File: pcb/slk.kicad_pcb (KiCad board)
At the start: 2 copper layers, 68.6 x 53.3 mm, 15 parts, among them J1 Screw Terminal, P1 Power, P2 Analog, P3 Digital 1, P4 Digital 2, U1 MCP2515-xSO, U2 TJA1055T1, Y1 Crystal

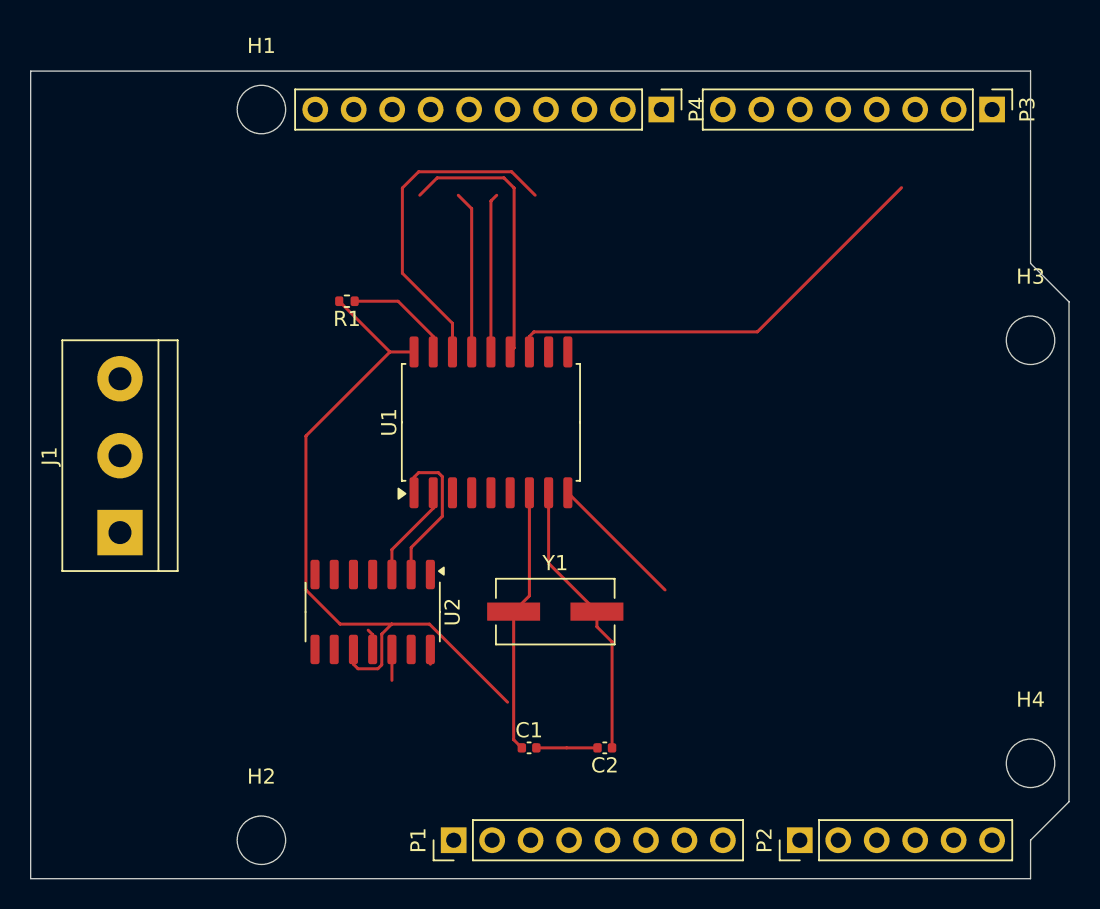
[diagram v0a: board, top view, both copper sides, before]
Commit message: it should work now
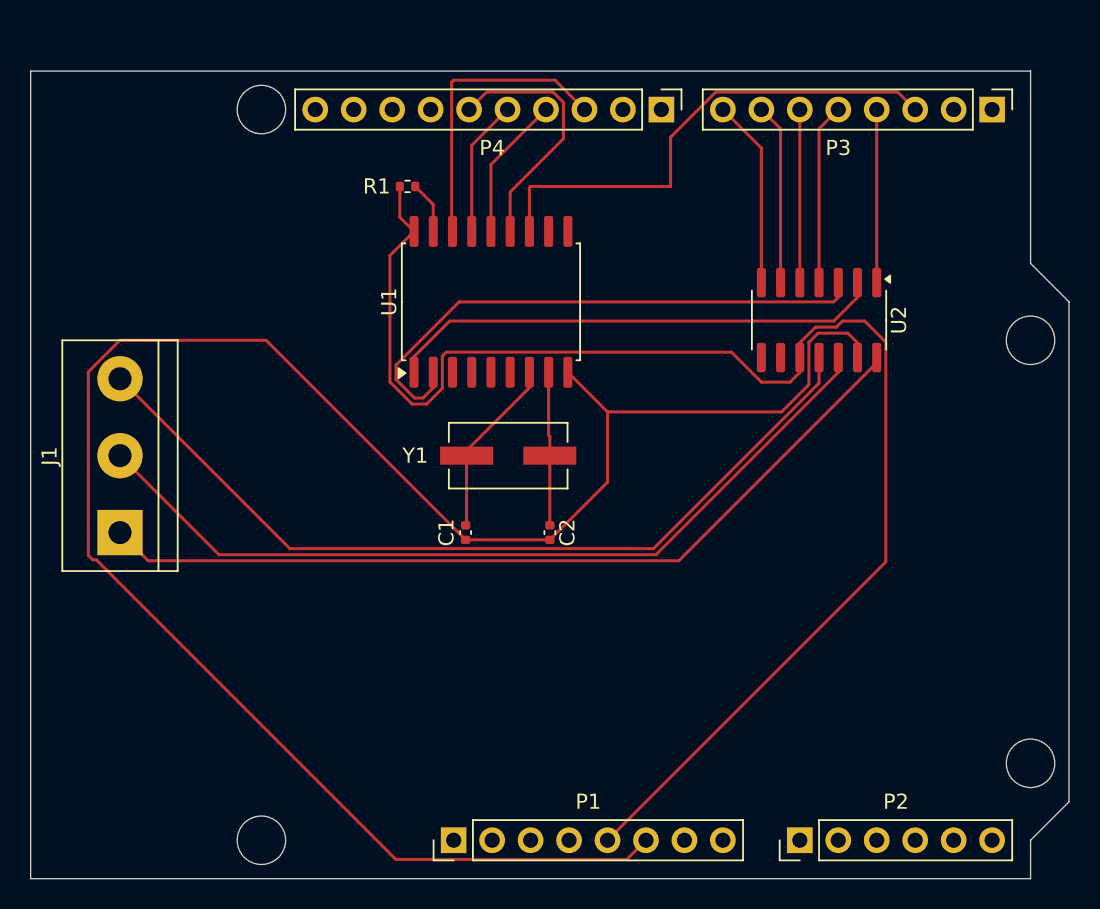
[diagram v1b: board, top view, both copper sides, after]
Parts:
- moved U2 35.2 mm to (153.7, 67.2)
- moved C1 14.8 mm to (130.3, 81.3), turned to -90 degrees
- moved C2 14.7 mm to (135.9, 81.3), turned to -90 degrees
- moved Y1 10.8 mm to (133.1, 76.2)
- moved R1 8.57 mm to (126.5, 58.4)
- moved U1 7.96 mm to (132.0, 66.0)
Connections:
- P3 pad 4: unconnected-(P3-Pin_4-Pad4) -> /INH
- P3 pad 5: unconnected-(P3-Pin_5-Pad5) -> /ERR
- P3 pad 6: unconnected-(P3-Pin_6-Pad6) -> /STB
- P3 pad 7: unconnected-(P3-Pin_7-Pad7) -> /EN
- P3 pad 8: unconnected-(P3-Pin_8-Pad8) -> /WAKE
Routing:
- net /GND: track 13.1 -> 129.9 mm
- net /CANH: track 1.40 -> 57.0 mm
- net /BAT+: track 0.97 -> 56.5 mm
- net /CANL: track 2.04 -> 56.1 mm
- net /5V: track 46.8 -> 94.7 mm
- net /RX: track 6.53 -> 37.3 mm
- net /TX: track 10.4 -> 32.9 mm
- net /WAKE: track 0.00 -> 12.5 mm
- net /ERR: track 0.00 -> 12.0 mm
- net /EN: track 0.00 -> 12.0 mm
- net /STB: track 0.00 -> 11.4 mm
- net /INH: track 0.00 -> 11.4 mm
- net Net-(U1-OSC1): track 18.6 -> 10.1 mm
- net Net-(U1-OSC2): track 17.5 -> 11.9 mm
- net Net-(U1-~{RESET}): track 7.18 -> 3.46 mm
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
